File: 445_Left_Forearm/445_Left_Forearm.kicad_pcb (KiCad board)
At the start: 2 copper layers, 24.9 x 18 mm, 2 parts, among them J1 69167-107HLF, U1 LSM6DSMTR

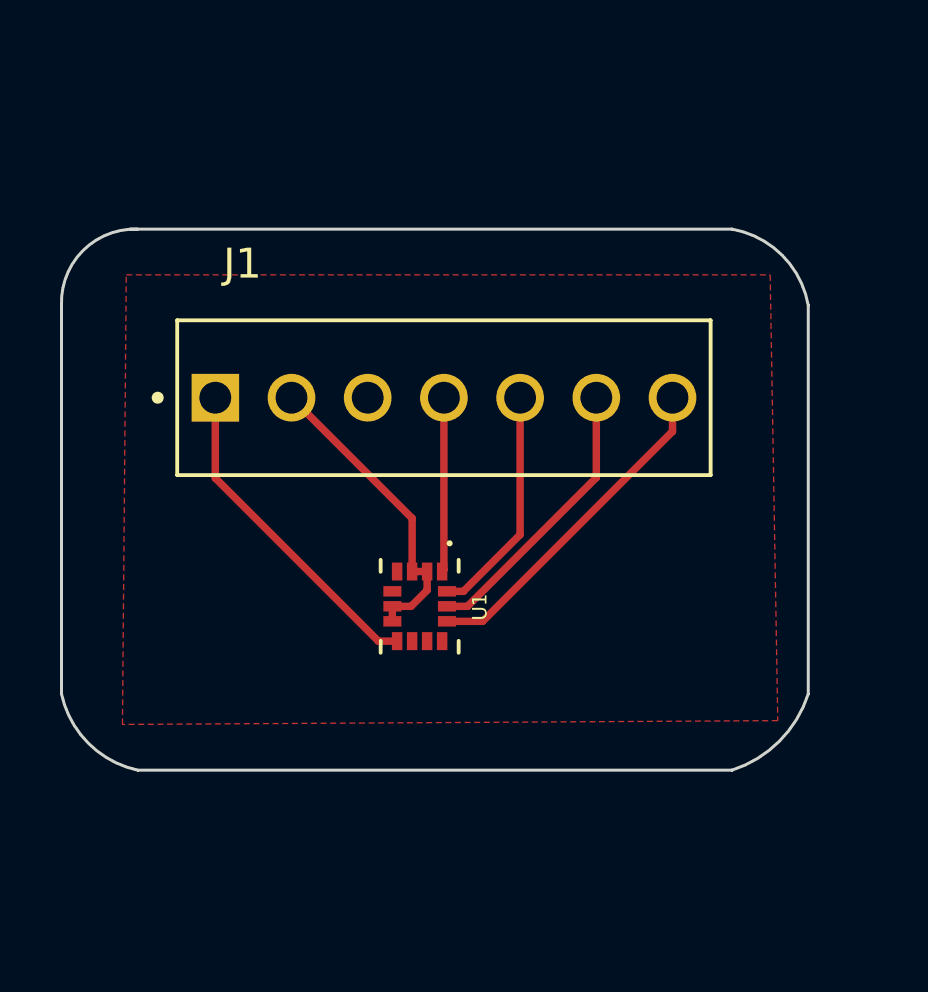
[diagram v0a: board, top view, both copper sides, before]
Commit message: Layout First Draft
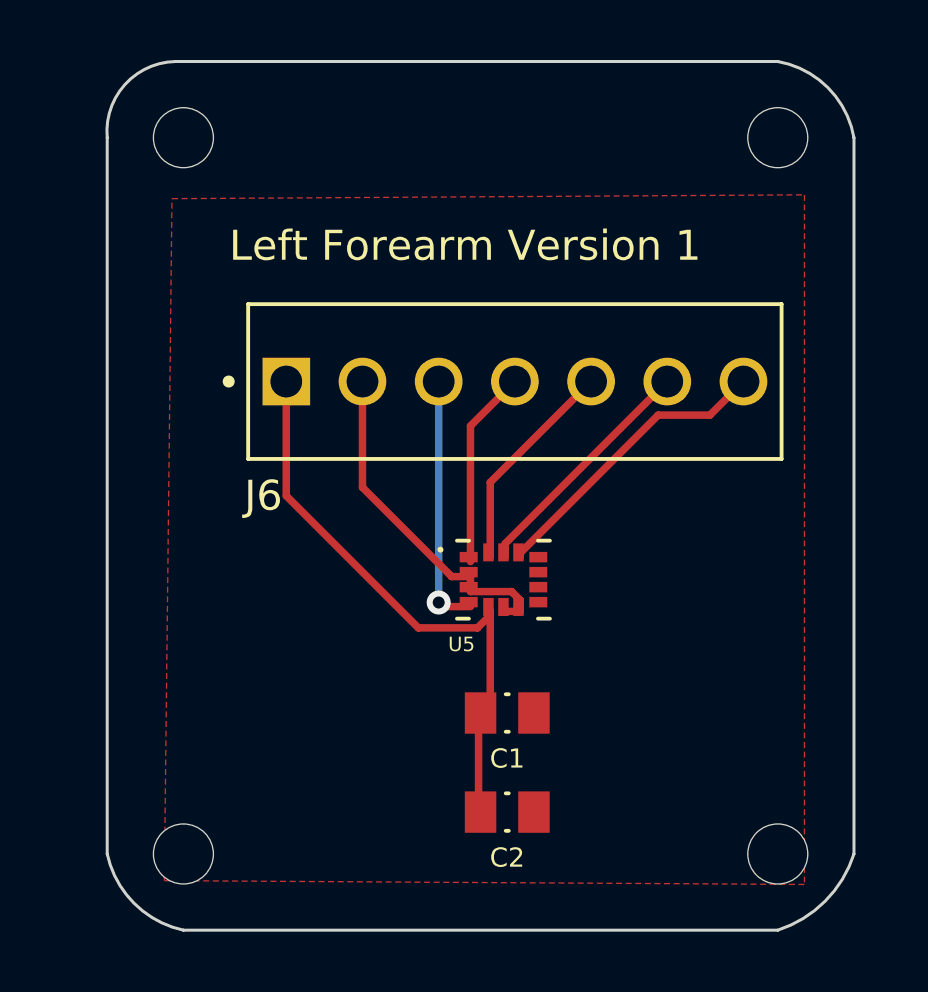
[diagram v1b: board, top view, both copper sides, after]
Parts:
- removed J1: 69167-107HLF, 69167-107HLF:AMPHENOL_69167-107HLF
- removed U1: LSM6DSMTR, LSM6DSMTR (1):PQFN50P300X250X86-14N
- added C1: 100nF, CL21F104ZAANNNC:CAPC2012X135N, F.Cu at (148.6, 94.6)
- added C2: 100nF, CL21F104ZAANNNC:CAPC2012X135N, F.Cu at (148.6, 97.9)
- added H1: MountingHole, MountingHole:MountingHole_2mm, F.Cu at (137.8, 75.4)
- added H2: MountingHole, MountingHole:MountingHole_2mm, F.Cu at (157.6, 75.4)
- added H3: MountingHole, MountingHole:MountingHole_2mm, F.Cu at (137.8, 99.3)
- added H4: MountingHole, MountingHole:MountingHole_2mm, F.Cu at (157.6, 99.3)
- added J6: 69167-107HLF, 69167-107HLF:AMPHENOL_69167-107HLF, F.Cu at (148.8, 83.6)
- added U5: LSM6DSMTR, LSM6DSMTR (1):PQFN50P300X250X86-14N, F.Cu at (148.5, 90.2)
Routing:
- net /CS2: track 11.3 -> 0.00 mm
- net /SENSOR_3: track 0.00 -> 9.93 mm
- net /CLK: track 9.42 -> 0.00 mm
- net /INT1_3: track 0.00 -> 8.48 mm, vias 0 -> 1
- net +3.3V: track 11.0 -> 19.4 mm
- net /CLK3: track 0.00 -> 8.08 mm
- net /MOSI: track 7.79 -> 0.00 mm
- net /MOSI_3: track 0.00 -> 7.23 mm
- net /MISO_3: track 0.00 -> 6.62 mm
- net /MISO: track 5.82 -> 0.00 mm
- net GND: track 10.5 -> 11.5 mm
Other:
- board size 24.9 x 18 mm -> 24.9 x 29 mm
- board text added: "Left Forearm Version 1"
